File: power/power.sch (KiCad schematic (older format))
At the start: 52 parts, among them J1 Conn_01x02_Female, J10 Conn_01x02_Female, J11 Conn_01x02_Female, J12 Conn_01x02_Female, J13 Conn_01x02_Female, J14 Conn_01x02_Female, J15 Conn_01x02_Female, J2 Barrel_jack, J3 CONN_02X03, J4 Conn_01x02_Female, J5 Conn_01x02_Female, J6 Conn_01x02_Female, J7 Conn_01x02_Female, J8 Conn_01x02_Female, J9 Conn_01x02_Female, Q1 BS170, Q2 BS170, Q3 BS170, Q5 BS170, Q6 BS170, Q7 BS170, U2 TPS2592xx, U3 ATMEGA16M1, U4 LP5907MFX-3_3_NOPB

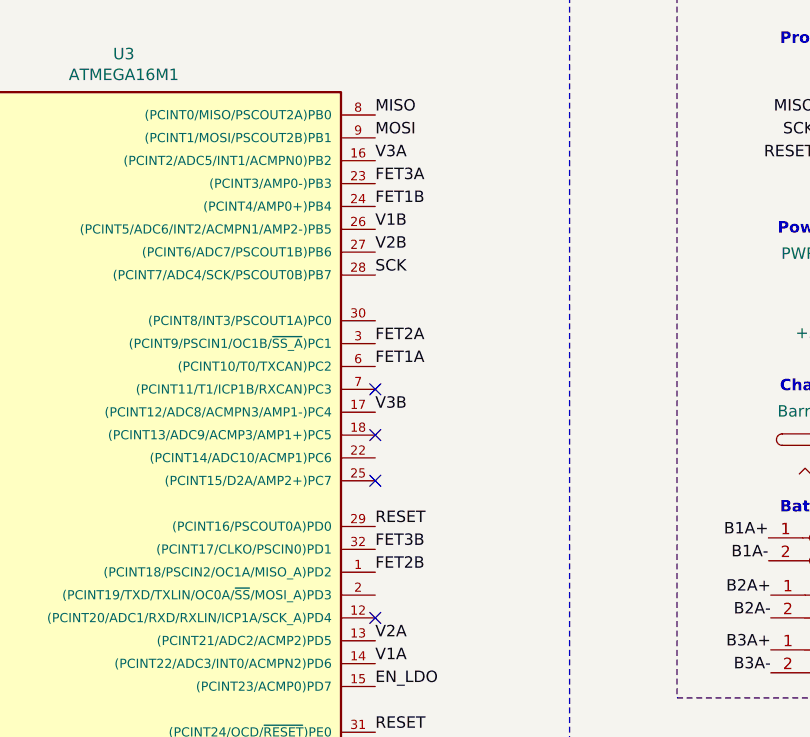
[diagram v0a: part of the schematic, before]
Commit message: half layout
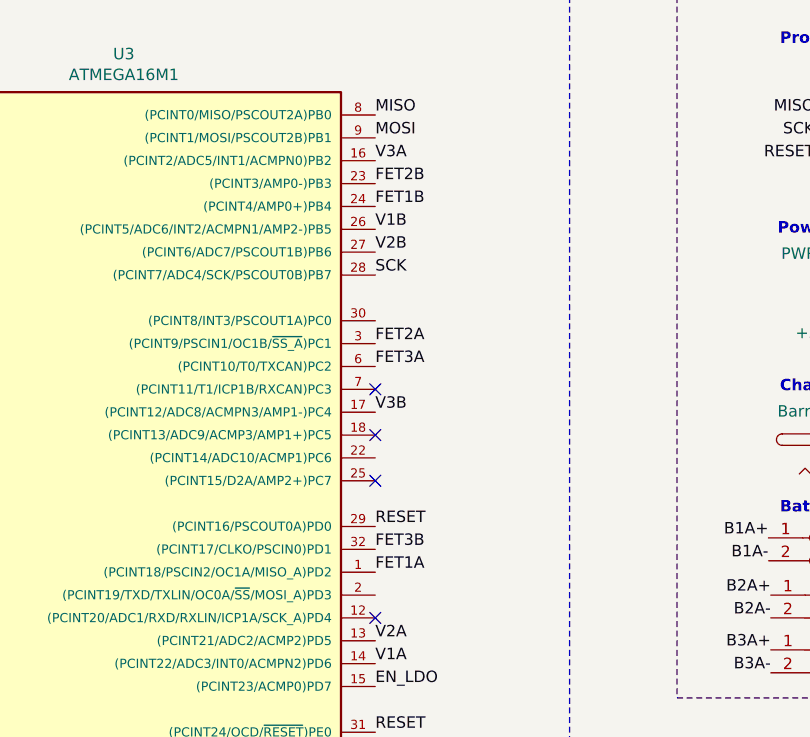
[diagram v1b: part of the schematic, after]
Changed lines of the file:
@@
 Text Label 870  8370 2    50   ~ 0
 BAT-
-Text Label 3740 2500 0    50   ~ 0
+Text Label 3740 3400 0    50   ~ 0
 FET1A
 Text Label 3740 2400 0    50   ~ 0
 FET2A
-Text Label 3740 1700 0    50   ~ 0
+Text Label 3740 2500 0    50   ~ 0
 FET3A
 Text Label 3740 1800 0    50   ~ 0
 FET1B
-Text Label 3740 3400 0    50   ~ 0
+Text Label 3740 1700 0    50   ~ 0
 FET2B
 Text Label 3740 3300 0    50   ~ 0

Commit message: complete layout
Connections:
- net labels removed: VCC
- no-connect marks 6 -> 8
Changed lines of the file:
@@
 MOSI
-$Comp
-L power:VCC #PWR0101
-U 1 1 5E15CCC8
-P 6310 1400
-F 0 "#PWR0101" H 6310 1250 50  0001 C CNN
-F 1 "VCC" H 6327 1573 50  0000 C CNN
-F 2 "" H 6310 1400 50  0001 C CNN
-F 3 "" H 6310 1400 50  0001 C CNN
-	1    6310 1400
-	1    0    0    -1
-$EndComp
 $Comp
 L power:GND #PWR0102
@@
 	1    0    0    -1
 $EndComp
-Text Label 3740 3700 0    50   ~ 0
+Text Label 3740 3500 0    50   ~ 0
 V2A
-Text Label 3740 1600 0    50   ~ 0
+Text Label 3740 2500 0    50   ~ 0
 V3A
-Text Label 3740 1900 0    50   ~ 0
+Text Label 3740 2000 0    50   ~ 0
 V1B
-Text Label 3740 2000 0    50   ~ 0
+Text Label 3740 3000 0    50   ~ 0
 V2B
-Text Label 3740 2700 0    50   ~ 0
+Text Label 3740 1700 0    50   ~ 0
 V3B
 Wire Wire Line
@@
 Text Label 3740 2400 0    50   ~ 0
 FET2A
-Text Label 3740 2500 0    50   ~ 0
+Text Label 3740 2600 0    50   ~ 0
 FET3A
+Text Label 3740 1900 0    50   ~ 0
+FET1B
 Text Label 3740 1800 0    50   ~ 0
-FET1B
-Text Label 3740 1700 0    50   ~ 0
 FET2B
-Text Label 3740 3300 0    50   ~ 0
+Text Label 3740 2900 0    50   ~ 0
 FET3B
 Text Label 870  5620 2    50   ~ 0
@@
 	3190 5620 3890 5620
 Connection ~ 3190 5620
-Text Label 3740 3800 0    50   ~ 0
+Text Label 3740 3300 0    50   ~ 0
 V1A
 $Comp
@@
 Wire Wire Line
 	1390 3900 1390 4000
-NoConn ~ 3740 2600
 NoConn ~ 3740 2800
-NoConn ~ 3740 3000
 NoConn ~ 3740 3600
 NoConn ~ 3740 4200
@@
 	0    1    1    0
 $EndComp
+NoConn ~ 3740 1600
+NoConn ~ 3740 2300
+NoConn ~ 3740 3700
+NoConn ~ 3740 3800
+$Comp
+L power:+3.3V #PWR?
+U 1 1 5FF49F28
+P 6310 1400
+F 0 "#PWR?" H 6310 1250 50  0001 C CNN
+F 1 "+3.3V" H 6325 1573 50  0000 C CNN
+F 2 "" H 6310 1400 50  0001 C CNN
+F 3 "" H 6310 1400 50  0001 C CNN
+	1    6310 1400
+	1    0    0    -1
+$EndComp
 $EndSCHEMATC
